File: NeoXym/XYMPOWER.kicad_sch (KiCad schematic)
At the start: 35 parts, among them J11 DE9_Receptacle, J12 DE9_Plug, J9 USB_B, U10 74HCT04, U15 74HCT00, U16 74HCT14, U19 MAX232, U21 CH340G, U4 74HCT32, U5 74HCT00, U6 74HCT09, U8 74HCT10, X2 12MHz

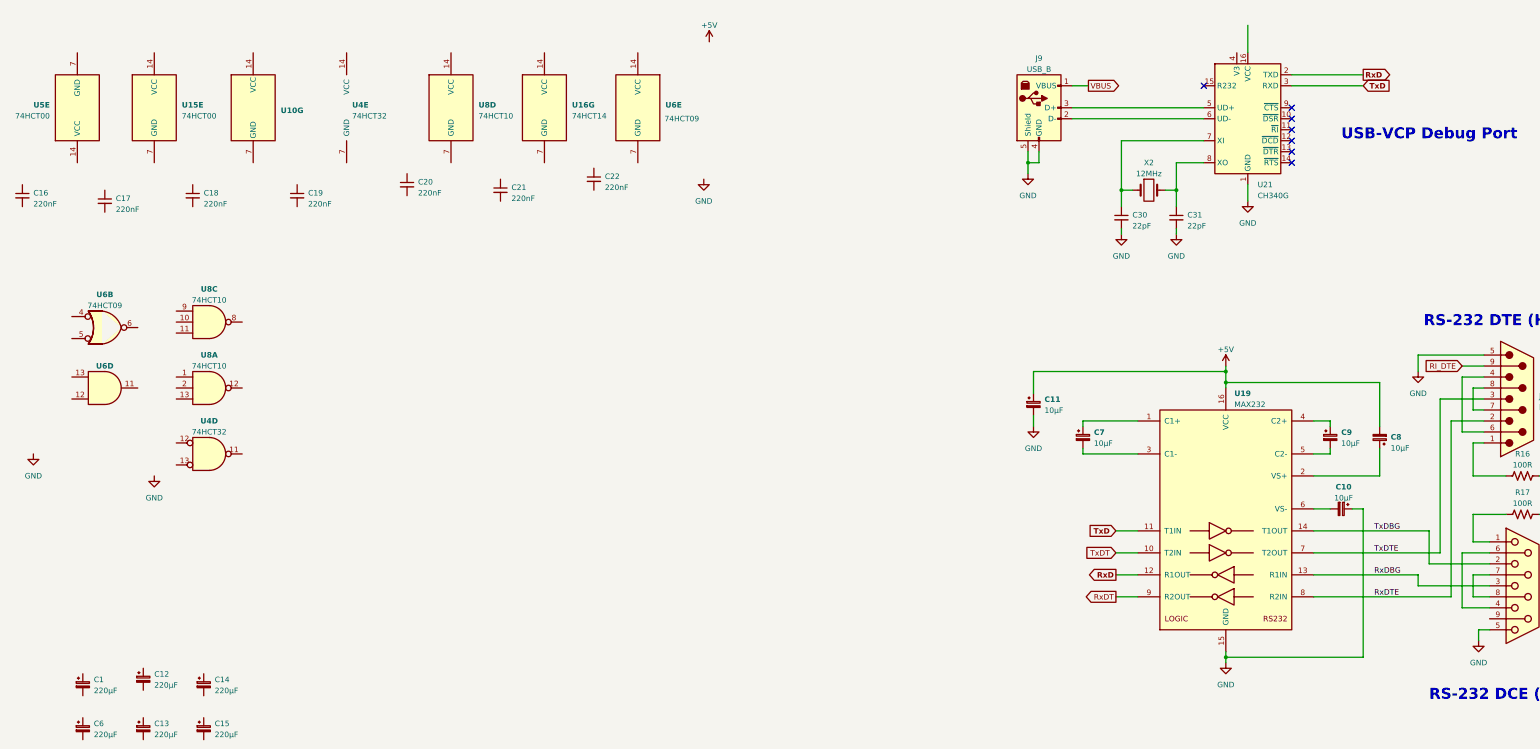
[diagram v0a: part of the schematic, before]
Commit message: modified:   CPU_MEM_IOCTRL.kicad_sch 	modified:   XYMGLUE.kicad_sch 	modified:   XYMPOWER.kicad_sch
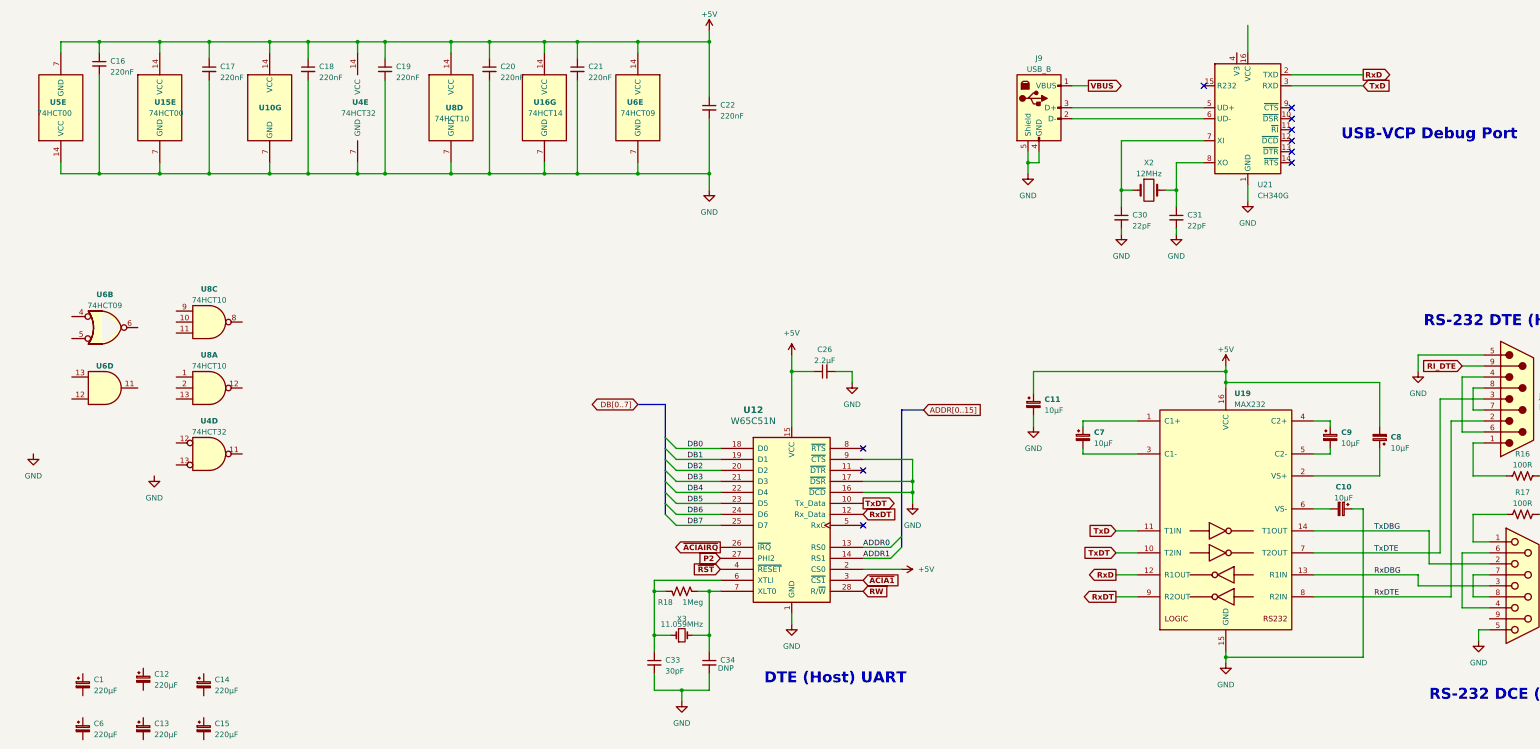
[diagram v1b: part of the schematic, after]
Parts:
- added C26: 2.2µF, symbol Device:C_Small
- added C33: 30pF, symbol Device:C_Small
- added C34: 18pF, symbol Device:C_Small
- added R18: 1Meg, symbol Device:R_US
- added U12: W65C51N, Package_DIP:DIP-28_W15.24mm_Socket, symbol 65xx:W65C51N
- added X3: 11.059MHz, symbol Device:Crystal_Small
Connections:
- net +5V: now also C16.1, C17.1, C18.1, C19.1, C20.1, C21.1, C22.1, U10.14 (VCC), U15.14 (VCC), U16.14 (VCC), U4.14 (VCC), U5.7 (GND), U6.14 (VCC), U8.14 (VCC), C26.1, U12.15 (VCC), U12.2 (CS0)
- net GND: now also C16.2, C17.2, C18.2, C19.2, C20.2, C21.2, C22.2, U10.7 (GND), U15.7 (GND), U16.7 (GND), U4.7 (GND), U5.14 (VCC), U6.7 (GND), U8.7 (GND), C26.2, C33.2, C34.2, U12.1 (GND), U12.16 (~{DCD}), U12.17 (~{DSR}), U12.9 (~{CTS})
- net RxDT: now also U12.12 (Rx_Data)
- net TxDT: now also U12.10 (Tx_Data)
- new net: C33.1, R18.1, U12.6 (XTLI), X3.1
- new net: C34.1, R18.2, U12.7 (XLT0), X3.2
- new net ADDR0: U12.13 (RS0)
- new net ADDR1: U12.14 (RS1)
- new net DB0: U12.18 (D0)
- new net DB1: U12.19 (D1)
- new net DB2: U12.20 (D2)
- new net DB3: U12.21 (D3)
- new net DB4: U12.22 (D4)
- new net DB5: U12.23 (D5)
- new net DB6: U12.24 (D6)
- new net DB7: U12.25 (D7)
- new net P2: U12.27 (PHI2)
- new net RW: U12.28 (R/~{W})
- new net ~{ACIA1}: U12.3 (~{CS1})
- new net ~{ACIAIRQ}: U12.26 (~{IRQ})
- new net ~{RST}: U12.4 (~{RESET})
- no-connect marks 7 -> 10
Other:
- note added: "DTE (Host) UART"
- moved on the sheet: C16, C17, C18, C19, C20, C21, C22, U10G, U15E, U4E, U5E
